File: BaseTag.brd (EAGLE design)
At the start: 25.4 x 25.4 mm, 50 parts, among them J1 PIN-1-10, J2 PIN-1-4, J3 PIN-1-4, J4 PIN-1-2, U1 BQ25504, U3 MSP430FR2512IPW16RSOIC

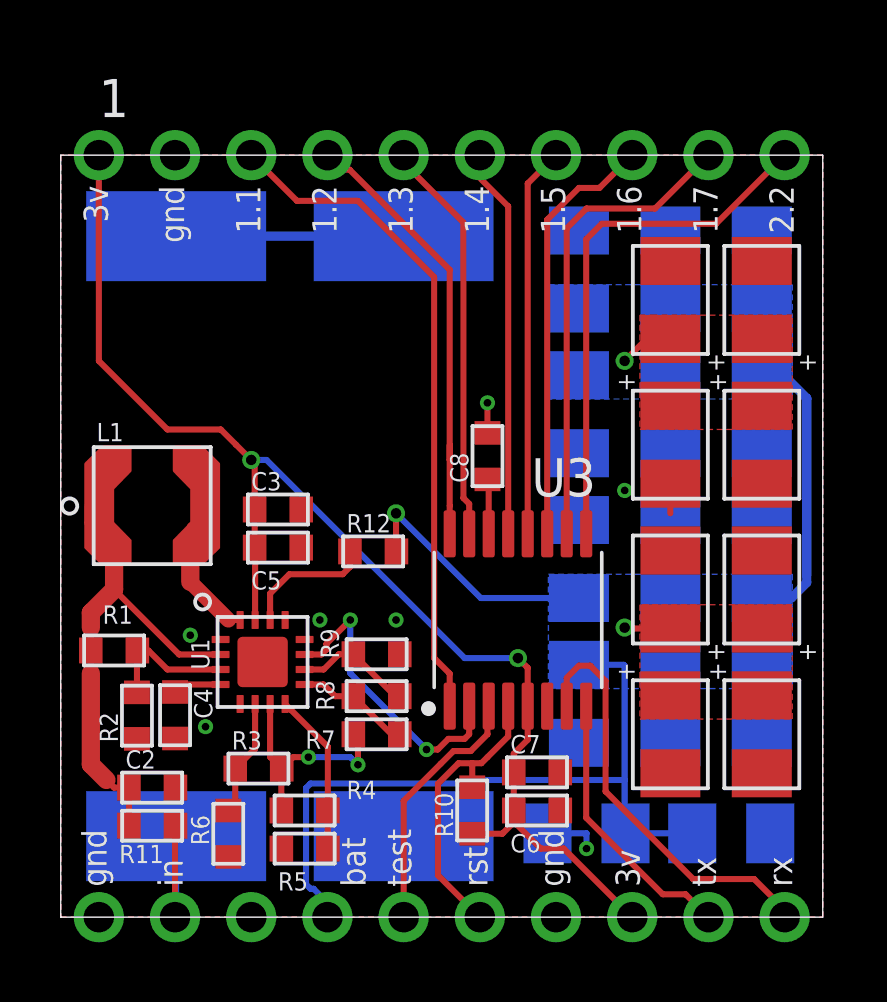
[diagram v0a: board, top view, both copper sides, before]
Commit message: v1 order
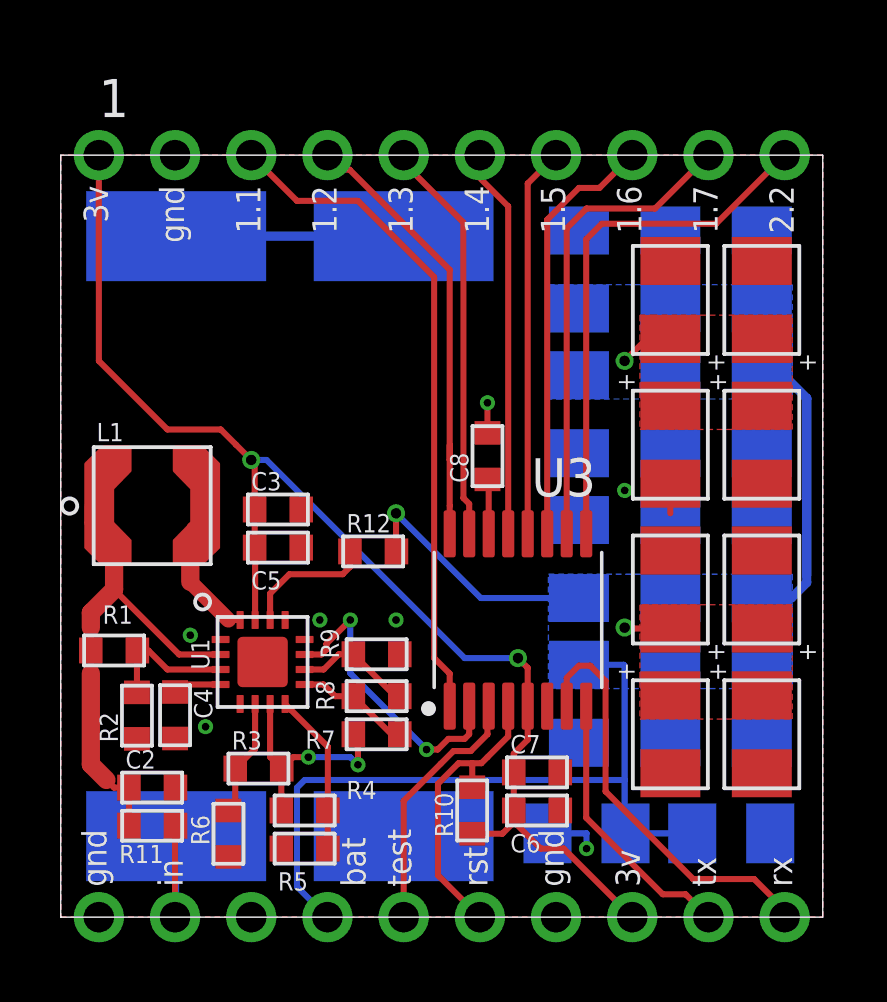
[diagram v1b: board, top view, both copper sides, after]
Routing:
- net VBAT: track 51.7 -> 52.4 mm
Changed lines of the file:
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@@
 <layer number="25" name="tNames" color="7" fill="1" visible="yes" active="yes"/>
 <layer number="26" name="bNames" color="7" fill="1" visible="yes" active="yes"/>
-<layer number="27" name="tValues" color="7" fill="1" visible="yes" active="yes"/>
-<layer number="28" name="bValues" color="7" fill="1" visible="yes" active="yes"/>
-<layer number="29" name="tStop" color="7" fill="3" visible="yes" active="yes"/>
-<layer number="30" name="bStop" color="7" fill="6" visible="yes" active="yes"/>
-<layer number="31" name="tCream" color="7" fill="4" visible="yes" active="yes"/>
-<layer number="32" name="bCream" color="7" fill="5" visible="yes" active="yes"/>
-<layer number="33" name="tFinish" color="6" fill="3" visible="yes" active="yes"/>
-<layer number="34" name="bFinish" color="6" fill="6" visible="yes" active="yes"/>
-<layer number="35" name="tGlue" color="7" fill="4" visible="yes" active="yes"/>
-<layer number="36" name="bGlue" color="7" fill="5" visible="yes" active="yes"/>
-<layer number="37" name="tTest" color="7" fill="1" visible="yes" active="yes"/>
-<layer number="38" name="bTest" color="7" fill="1" visible="yes" active="yes"/>
+<layer number="27" name="tValues" color="7" fill="1" visible="no" active="yes"/>
+<layer number="28" name="bValues" color="7" fill="1" visible="no" active="yes"/>
+<layer number="29" name="tStop" color="7" fill="3" visible="no" active="yes"/>
+<layer number="30" name="bStop" color="7" fill="6" visible="no" active="yes"/>
+<layer number="31" name="tCream" color="7" fill="4" visible="no" active="yes"/>
+<layer number="32" name="bCream" color="7" fill="5" visible="no" active="yes"/>
+<layer number="33" name="tFinish" color="6" fill="3" visible="no" active="yes"/>
+<layer number="34" name="bFinish" color="6" fill="6" visible="no" active="yes"/>
+<layer number="35" name="tGlue" color="7" fill="4" visible="no" active="yes"/>
+<layer number="36" name="bGlue" color="7" fill="5" visible="no" active="yes"/>
+<layer number="37" name="tTest" color="7" fill="1" visible="no" active="yes"/>
+<layer number="38" name="bTest" color="7" fill="1" visible="no" active="yes"/>
 <layer number="39" name="tKeepout" color="4" fill="11" visible="yes" active="yes"/>
 <layer number="40" name="bKeepout" color="1" fill="11" visible="yes" active="yes"/>
 <layer number="41" name="tRestrict" color="4" fill="10" visible="yes" active="yes"/>
 <layer number="42" name="bRestrict" color="1" fill="10" visible="yes" active="yes"/>
-<layer number="43" name="vRestrict" color="2" fill="10" visible="yes" active="yes"/>
-<layer number="44" name="Drills" color="7" fill="1" visible="yes" active="yes"/>
-<layer number="45" name="Holes" color="7" fill="1" visible="yes" active="yes"/>
-<layer number="46" name="Milling" color="3" fill="1" visible="yes" active="yes"/>
-<layer number="47" name="Measures" color="7" fill="1" visible="yes" active="yes"/>
-<layer number="48" name="Document" color="7" fill="1" visible="yes" active="yes"/>
-<layer number="49" name="Reference" color="7" fill="1" visible="yes" active="yes"/>
+<layer number="43" name="vRestrict" color="2" fill="10" visible="no" active="yes"/>
+<layer number="44" name="Drills" color="7" fill="1" visible="no" active="yes"/>
+<layer number="45" name="Holes" color="7" fill="1" visible="no" active="yes"/>
+<layer number="46" name="Milling" color="3" fill="1" visible="no" active="yes"/>
+<layer number="47" name="Measures" color="7" fill="1" visible="no" active="yes"/>
+<layer number="48" name="Document" color="7" fill="1" visible="no" active="yes"/>
+<layer number="49" name="Reference" color="7" fill="1" visible="no" active="yes"/>
 <layer number="51" name="tDocu" color="7" fill="1" visible="yes" active="yes"/>
 <layer number="52" name="bDocu" color="7" fill="1" visible="yes" active="yes"/>
@@
 <param name="mlMinCreamFrame" value="0mil"/>
 <param name="mlMaxCreamFrame" value="0mil"/>
-<param name="mlViaStopLimit" value="0mil"/>
+<param name="mlViaStopLimit" value="11mil"/>
 <param name="srRoundness" value="0"/>
 <param name="srMinRoundness" value="0mil"/>
@@
 <wire x1="19.528" y1="19.274" x2="18.796" y2="18.542" width="0.2032" layer="1"/>
 <via x="18.796" y="18.542" extent="1-16" drill="0.35"/>
-<wire x1="13.344" y1="4.454" x2="13.462" y2="4.572" width="0.2032" layer="16"/>
-<wire x1="8.3247875" y1="4.454" x2="13.344" y2="4.454" width="0.2032" layer="16"/>
-<wire x1="8.3247875" y1="4.454" x2="8.176" y2="4.3052125" width="0.2032" layer="16"/>
-<wire x1="8.176" y1="4.3052125" x2="8.176" y2="3.556" width="0.2032" layer="16"/>
-<wire x1="8.176" y1="3.556" x2="8.176" y2="1.0947875" width="0.2032" layer="16"/>
-<wire x1="8.176" y1="1.0947875" x2="8.3247875" y2="0.946" width="0.2032" layer="16"/>
-<wire x1="8.3247875" y1="0.946" x2="8.4266" y2="0.946" width="0.2032" layer="16"/>
-<wire x1="8.4266" y1="0.946" x2="8.89" y2="0.4826" width="0.2032" layer="16"/>
-<wire x1="18.796" y1="4.572" x2="13.462" y2="4.572" width="0.2032" layer="16"/>
 <wire x1="18.796" y1="4.572" x2="18.796" y2="8.382" width="0.2032" layer="16"/>
 <wire x1="18.796" y1="8.382" x2="18.766" y2="8.412" width="0.2032" layer="16"/>
 <wire x1="18.766" y1="8.412" x2="17.272" y2="8.412" width="0.2032" layer="16"/>
 <wire x1="24.8666" y1="11.4046" x2="24.8666" y2="17.2974" width="0.3048" layer="16"/>
+<wire x1="8.128" y1="4.572" x2="7.874" y2="4.318" width="0.2032" layer="16"/>
+<wire x1="7.874" y1="4.318" x2="7.874" y2="1.016" width="0.2032" layer="16"/>
+<wire x1="7.874" y1="1.016" x2="8.4074" y2="0.4826" width="0.2032" layer="16"/>
+<wire x1="8.4074" y1="0.4826" x2="8.89" y2="0.4826" width="0.2032" layer="16"/>
+<wire x1="18.796" y1="4.572" x2="8.128" y2="4.572" width="0.2032" layer="16"/>
 <wire x1="8.89" y1="0.4826" x2="8.89" y2="0" width="0" layer="19" extent="16-16"/>
 </signal>
